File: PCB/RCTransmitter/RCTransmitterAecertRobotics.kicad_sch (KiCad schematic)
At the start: 41 parts, among them J5019_1 J5019 Charger, K1 KCD1 Power Switch, P1 PCF8575

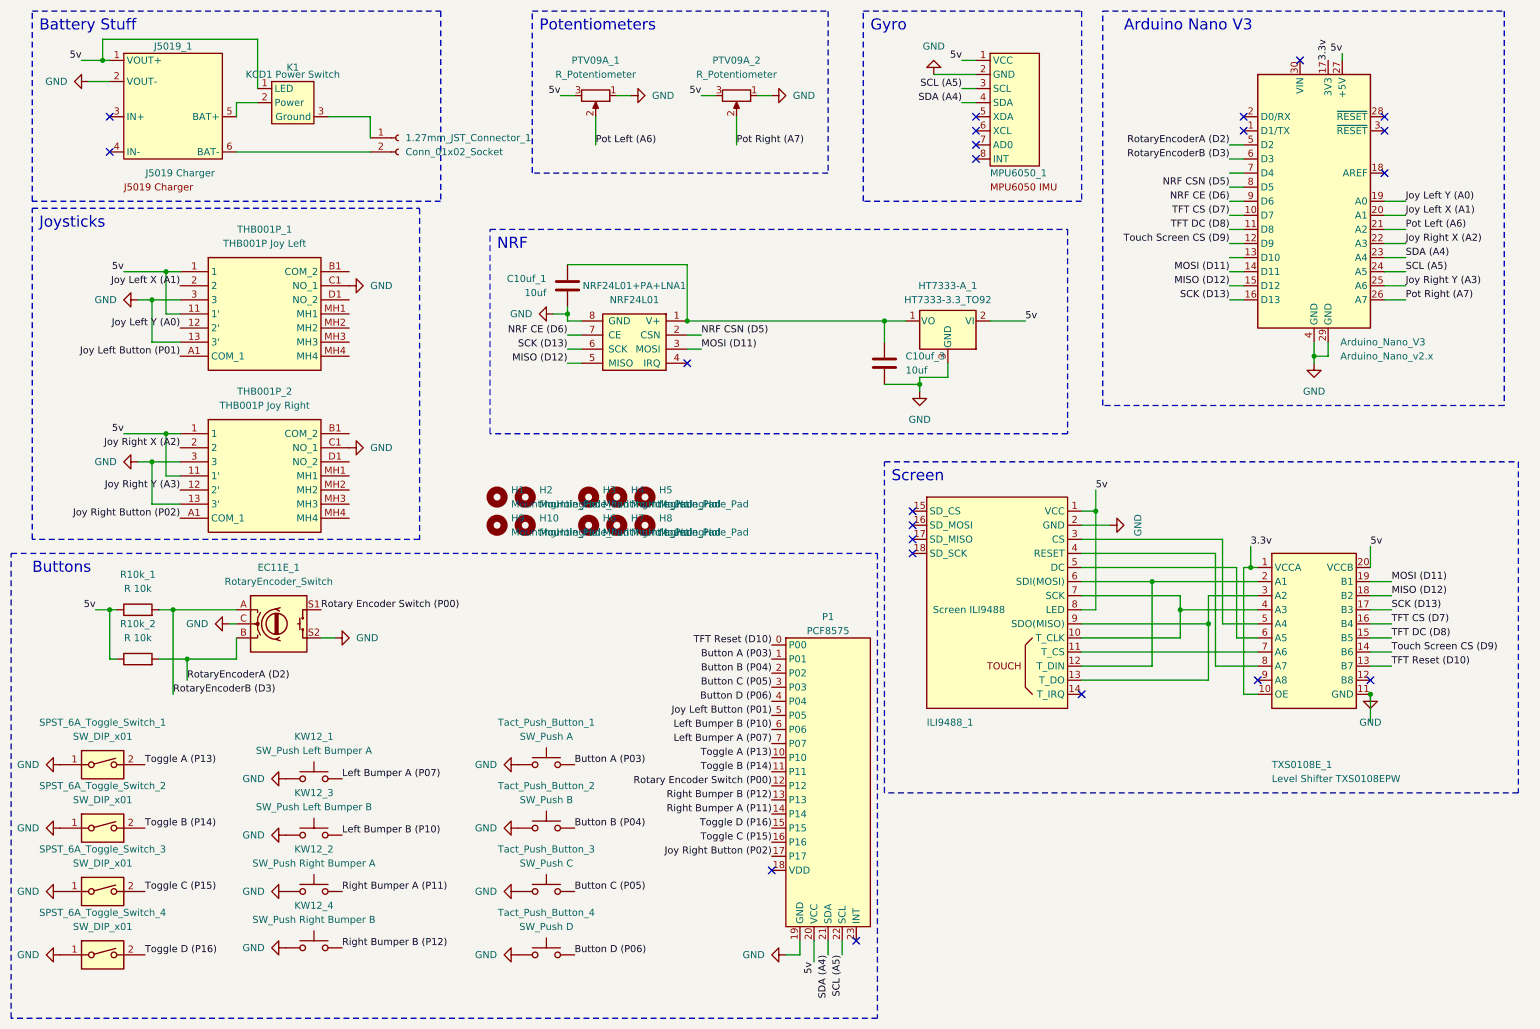
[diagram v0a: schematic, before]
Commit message: updated new design
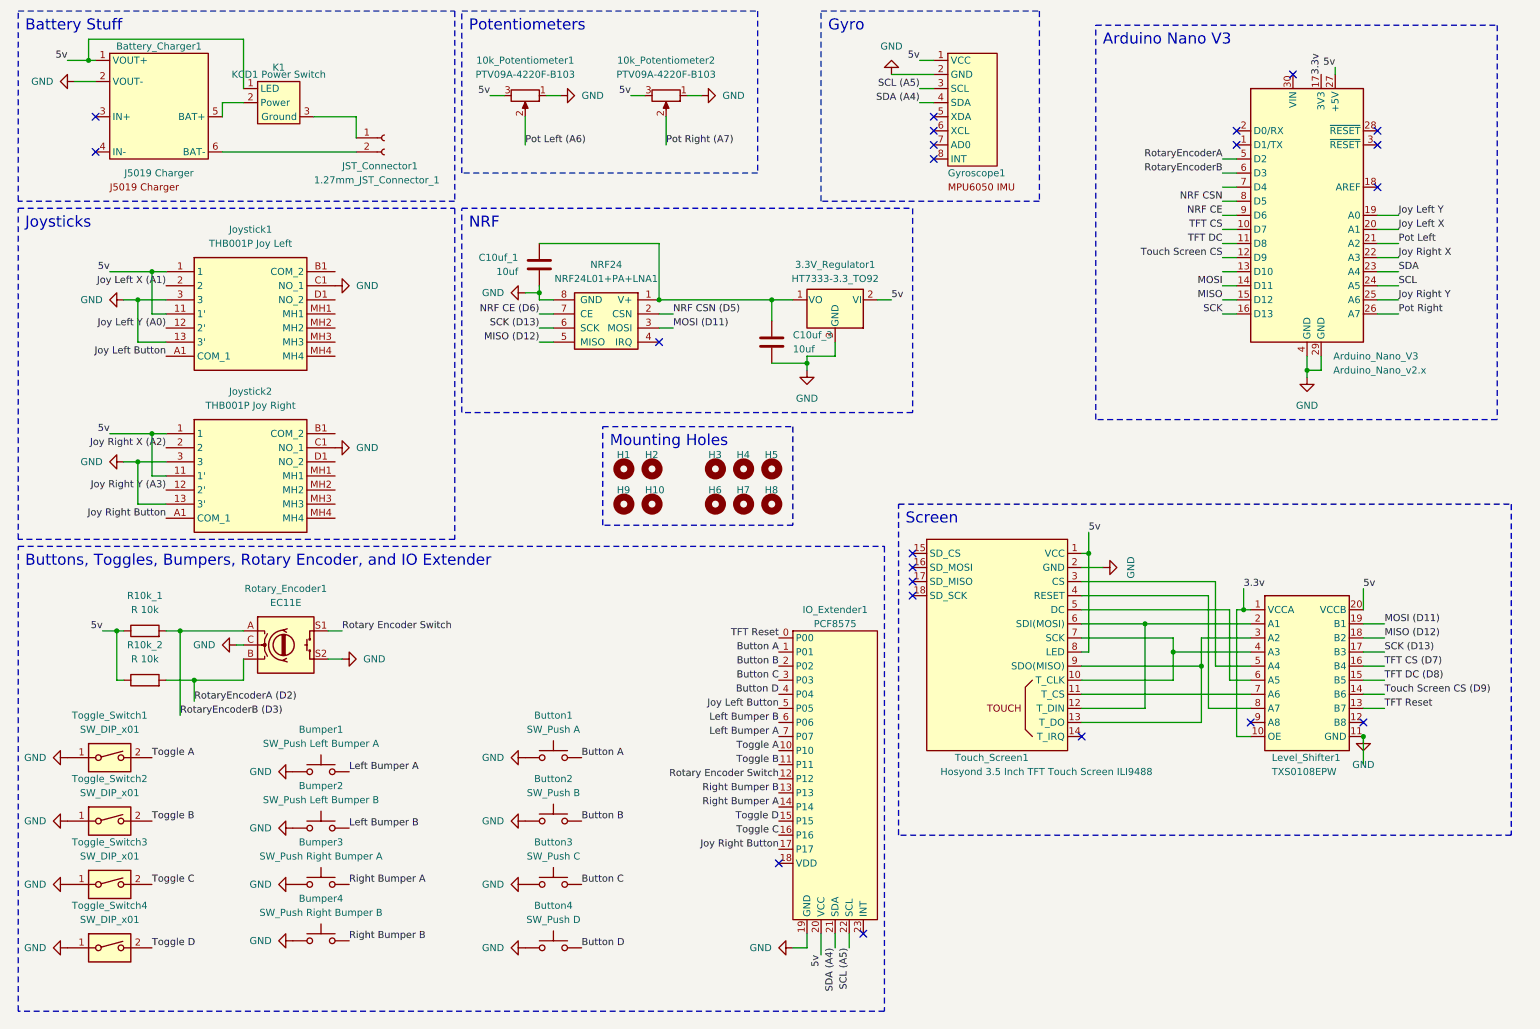
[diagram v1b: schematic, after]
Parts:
- 10k_Potentiometer1: renamed from ‎PTV09A_1; value R_Potentiometer -> PTV09A-4220F-B103
- 10k_Potentiometer2: renamed from ‎PTV09A_2; value R_Potentiometer -> PTV09A-4220F-B103
- JST_Connector1: renamed from 1.27mm_JST_Connector_1; value Conn_01x02_Socket -> 1.27mm_JST_Connector_1
- Level_Shifter1: renamed from TXS0108E_1; value Level Shifter TXS0108EPW -> TXS0108EPW
- NRF24: renamed from NRF24L01+PA+LNA1; value NRF24L01 -> NRF24L01+PA+LNA1
- Rotary_Encoder1: renamed from EC11E_1; value RotaryEncoder_Switch -> EC11E
- Touch_Screen1: renamed from ILI9488_1; value Screen ILI9488 -> Hosyond 3.5 Inch TFT Touch Screen ILI9488
- renumbered HT7333-A_1 to 3.3V_Regulator1, J5019_1 to Battery_Charger1, KW12_1 to Bumper1, KW12_3 to Bumper2, KW12_2 to Bumper3, KW12_4 to Bumper4, Tact_Push_Button_1 to Button1, Tact_Push_Button_2 to Button2, Tact_Push_Button_3 to Button3, Tact_Push_Button_4 to Button4, MPU6050_1 to Gyroscope1, P1 to IO_Extender1, THB001P_1 to Joystick1, THB001P_2 to Joystick2, SPST_6A_Toggle_Switch_1 to Toggle_Switch1, SPST_6A_Toggle_Switch_2 to Toggle_Switch2, SPST_6A_Toggle_Switch_3 to Toggle_Switch3, SPST_6A_Toggle_Switch_4 to Toggle_Switch4
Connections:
- net Joy Left X (A1): no longer Arduino_Nano_V3.20 (A1)
- net Joy Left Y (A0): no longer Arduino_Nano_V3.19 (A0)
- net Joy Right X (A2): no longer Arduino_Nano_V3.22 (A3)
- net Joy Right Y (A3): no longer Arduino_Nano_V3.25 (A6)
- net MISO (D12): no longer Arduino_Nano_V3.15 (D12)
- net MOSI (D11): no longer Arduino_Nano_V3.14 (D11)
- net NRF CE (D6): no longer Arduino_Nano_V3.9 (D6)
- net NRF CSN (D5): no longer Arduino_Nano_V3.8 (D5)
- net Pot Left (A6): no longer Arduino_Nano_V3.21 (A2)
- net Pot Right (A7): no longer Arduino_Nano_V3.26 (A7)
- net RotaryEncoderA (D2): no longer Arduino_Nano_V3.5 (D2)
- net RotaryEncoderB (D3): no longer Arduino_Nano_V3.6 (D3)
- net SCK (D13): no longer Arduino_Nano_V3.16 (D13)
- net SCL (A5): no longer Arduino_Nano_V3.24 (A5)
- net SDA (A4): no longer Arduino_Nano_V3.23 (A4)
- net TFT CS (D7): no longer Arduino_Nano_V3.10 (D7)
- net TFT DC (D8): no longer Arduino_Nano_V3.11 (D8)
- net Touch Screen CS (D9): no longer Arduino_Nano_V3.12 (D9)
- net Button A (P03) renamed Button A
- net Button B (P04) renamed Button B
- net Button C (P05) renamed Button C
- net Button D (P06) renamed Button D
- net Joy Left Button (P01) renamed Joy Left Button
- net Joy Right Button (P02) renamed Joy Right Button
- net Left Bumper A (P07) renamed Left Bumper A
- net Left Bumper B (P10) renamed Left Bumper B
- net Right Bumper A (P11) renamed Right Bumper A
- net Right Bumper B (P12) renamed Right Bumper B
- net Rotary Encoder Switch (P00) renamed Rotary Encoder Switch
- net TFT Reset (D10) renamed TFT Reset
- net Toggle A (P13) renamed Toggle A
- net Toggle B (P14) renamed Toggle B
- net Toggle C (P15) renamed Toggle C
- net Toggle D (P16) renamed Toggle D
- new net Joy Left X: Arduino_Nano_V3.20 (A1)
- new net Joy Left Y: Arduino_Nano_V3.19 (A0)
- new net Joy Right X: Arduino_Nano_V3.22 (A3)
- new net Joy Right Y: Arduino_Nano_V3.25 (A6)
- new net MISO: Arduino_Nano_V3.15 (D12)
- new net MOSI: Arduino_Nano_V3.14 (D11)
- new net NRF CE: Arduino_Nano_V3.9 (D6)
- new net NRF CSN: Arduino_Nano_V3.8 (D5)
- new net Pot Left: Arduino_Nano_V3.21 (A2)
- new net Pot Right: Arduino_Nano_V3.26 (A7)
- new net RotaryEncoderA: Arduino_Nano_V3.5 (D2)
- new net RotaryEncoderB: Arduino_Nano_V3.6 (D3)
- new net SCK: Arduino_Nano_V3.16 (D13)
- new net SCL: Arduino_Nano_V3.24 (A5)
- new net SDA: Arduino_Nano_V3.23 (A4)
- new net TFT CS: Arduino_Nano_V3.10 (D7)
- new net TFT DC: Arduino_Nano_V3.11 (D8)
- new net Touch Screen CS: Arduino_Nano_V3.12 (D9)
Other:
- note added: "Buttons, Toggles, Bumpers, Rotary Encoder, and IO Extender"
- note added: "Mounting Holes"
- note removed: "Buttons"
- company: (none) -> Aecert Robotics 
- title: (none) -> Arduino Nano Powered RC Transmitter
- moved on the sheet: 10k_Potentiometer1, 10k_Potentiometer2, 3.3V_Regulator1, Arduino_Nano_V3, Battery_Charger1, Bumper1, Bumper2, Bumper3, Bumper4, Button1, Button2, Button3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
